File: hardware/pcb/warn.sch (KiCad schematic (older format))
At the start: 16 parts, among them CON2 MMCX_CONN, Q1 Q_NPN_BEC, U8 TPS61041, U9 ZXMHC6A07N8

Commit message: hw fixes
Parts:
- Q1: symbol Q_NPN_BEC -> Q_NPN_BEC-RESCUE-aero
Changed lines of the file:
@@
 Confirm pin assignments of NPN
 $Comp
-L Q_NPN_BEC Q1
+L Q_NPN_BEC-RESCUE-aero Q1
 U 1 1 5546CD30
 P 7750 5650

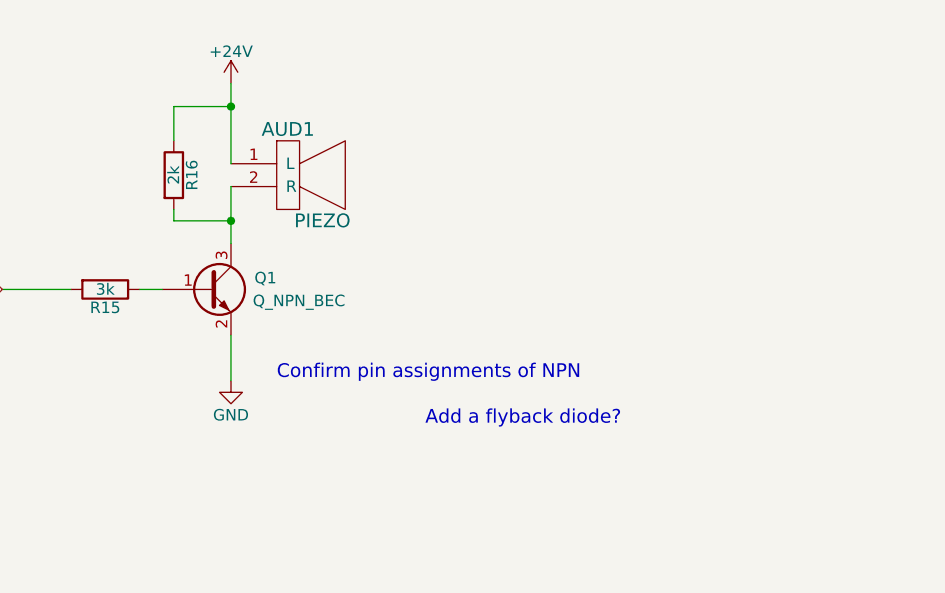
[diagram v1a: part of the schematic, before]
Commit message: committing hardware updates (probably unnecessary)
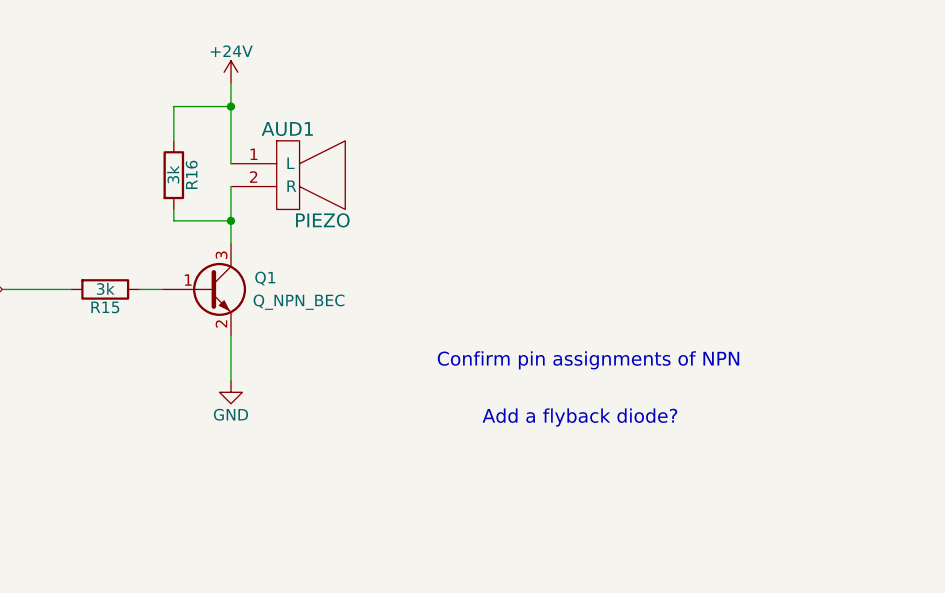
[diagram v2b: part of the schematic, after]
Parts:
- R16: value 2k -> 3k
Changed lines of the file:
@@
 P 7600 5150
 F 0 "R16" V 7680 5150 50  0000 C CNN
-F 1 "2k" V 7600 5150 50  0000 C CNN
+F 1 "3k" V 7600 5150 50  0000 C CNN
 F 2 "Resistors_SMD:R_0603" V 7530 5150 30  0001 C CNN
 F 3 "" H 7600 5150 30  0000 C CNN
@@
 Text Notes 2500 2600 0    60   ~ 0
 NOTE: Update R when LED is picked out
-Text Notes 8700 6250 0    60   ~ 0
+Text Notes 8950 6250 0    60   ~ 0
 Add a flyback diode?
 $Comp
@@
 	1    0    0    -1
 $EndComp
-Text Notes 8050 6050 0    60   ~ 0
+Text Notes 8750 6000 0    60   ~ 0
 Confirm pin assignments of NPN
 $Comp
